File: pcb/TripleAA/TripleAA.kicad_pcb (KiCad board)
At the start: 2 copper layers, 16 x 20 mm, 12 parts, among them J2 JST_S2B-PH-SM4-x, U2 TPS562242

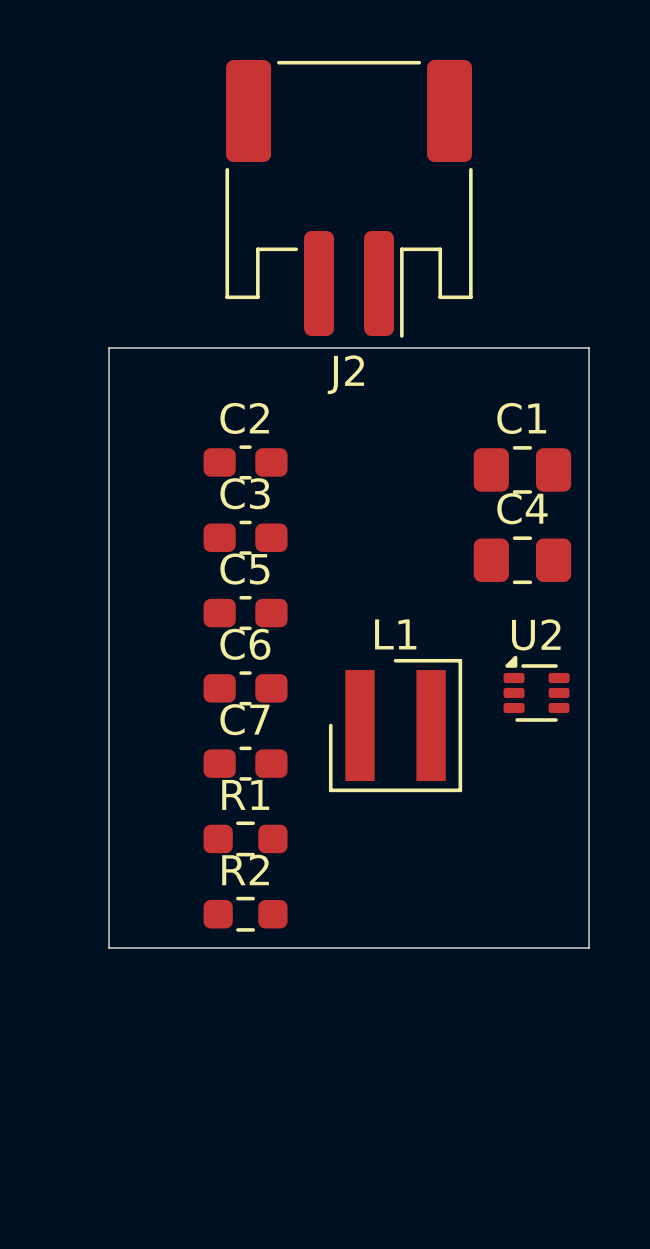
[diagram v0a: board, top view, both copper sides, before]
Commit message: Update SCH and PCB
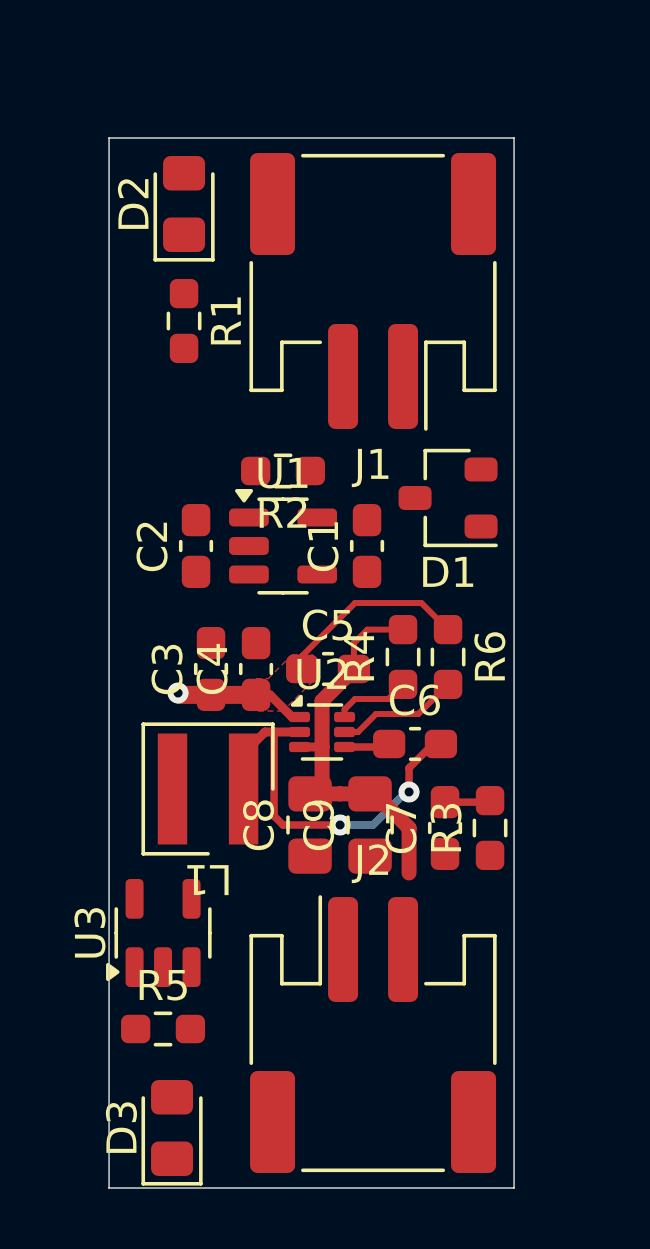
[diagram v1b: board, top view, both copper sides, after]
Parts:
- added C1: 10uF,25V,X5R,0603, Capacitor_SMD:C_0603_1608Metric_Pad1.08x0.95mm_HandSolder, F.Cu at (98.6, 61.6)
- added C2: 10uF,25V,X5R,0603, Capacitor_SMD:C_0603_1608Metric_Pad1.08x0.95mm_HandSolder, F.Cu at (92.9, 61.6)
- added D1: 824021, Package_TO_SOT_SMD_User:SOT-23_Handsoldering, F.Cu at (101.3, 60.0)
- added D2: 150080GS75000, LED_SMD:LED_0805_2012Metric_Pad1.15x1.40mm_HandSolder, F.Cu at (92.5, 50.2)
- added D3: 150080SS75000, LED_SMD:LED_0805_2012Metric_Pad1.15x1.40mm_HandSolder, F.Cu at (92.1, 81.0)
- added J1: JST_S2B-PH-SM4-x, Connector_User:JST_PH_S2B-PH-SM4-TB_1x02-1MP_P2.00mm_Horizontal, F.Cu at (98.8, 53.1)
- added R1: 2k,0603, Resistor_SMD:R_0603_1608Metric_Pad0.98x0.95mm_HandSolder, F.Cu at (92.5, 54.1)
- added R2: 2k,0603, Resistor_SMD:R_0603_1608Metric_Pad0.98x0.95mm_HandSolder, F.Cu at (95.8, 59.1)
- added R5: 27.4k,0603, Resistor_SMD:R_0603_1608Metric_Pad0.98x0.95mm_HandSolder, F.Cu at (91.8, 77.7)
- added R6: 10k,0603, Resistor_SMD:R_0603_1608Metric_Pad0.98x0.95mm_HandSolder, F.Cu at (101.3, 65.3)
- added U1: MCP73831-2-OT, Package_TO_SOT_SMD:SOT-23-5, F.Cu at (95.8, 61.6)
- added U3: BD4836G-xx, Package_TO_SOT_SMD:SOT-23-5, F.Cu at (91.8, 74.5)
- L1: value 74438357068 -> 74438356056; footprint Inductor_SMD_User:L_Wurth_WE-MAPI-4030 -> Inductor_SMD_User:L_Wurth_WE-MAPI-4020
- moved J2 27.9 mm to (98.8, 77.9), turned to 0 degrees
- moved C8 13.8 mm to (96.7, 70.9), turned to 90 degrees
- moved C9 10.2 mm to (98.7, 70.9), turned to 90 degrees
- moved R4 10.1 mm to (99.8, 65.3), turned to 90 degrees
- moved R3 8.16 mm to (102.7, 71.0), turned to 90 degrees
- moved C7 8.12 mm to (101.2, 71.0), turned to 90 degrees
- moved U2 7.27 mm to (97.1, 67.8)
- moved C6 7.14 mm to (100.2, 68.2)
- moved C4 6.89 mm to (94.9, 65.7), turned to 90 degrees
- moved L1 6.60 mm to (93.3, 69.7), turned to 180 degrees
- moved C3 4.52 mm to (93.4, 65.7), turned to 90 degrees
- moved C5 4.19 mm to (97.3, 65.7)
- renumbered C2 to C4, C7 to C5, C5 to C6, C6 to C7, C1 to C8, C4 to C9, R1 to R3, R2 to R4
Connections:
- U2 pad 5: +BATT -> Net-(U2-EN)
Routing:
- net /-Vout: track 0.00 -> 14.0 mm
- net Net-(U2-SW): track 0.00 -> 13.4 mm, vias 0 -> 2
- net +BATT: track 0.00 -> 10.9 mm, vias 0 -> 1
- net Net-(U2-EN): track 0.00 -> 4.11 mm
- net Net-(U2-FB): track 0.00 -> 3.84 mm
- net Net-(U2-BST): track 0.00 -> 1.53 mm
- added copper zone on F.Cu, net +BATT
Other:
- board size 16 x 20 mm -> 13.5 x 35 mm
